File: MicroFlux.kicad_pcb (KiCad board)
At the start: 2 copper layers, 30.5 x 53.3 mm, 24 parts, among them J1 Audio Out, J2 Audio In, U1 LM358

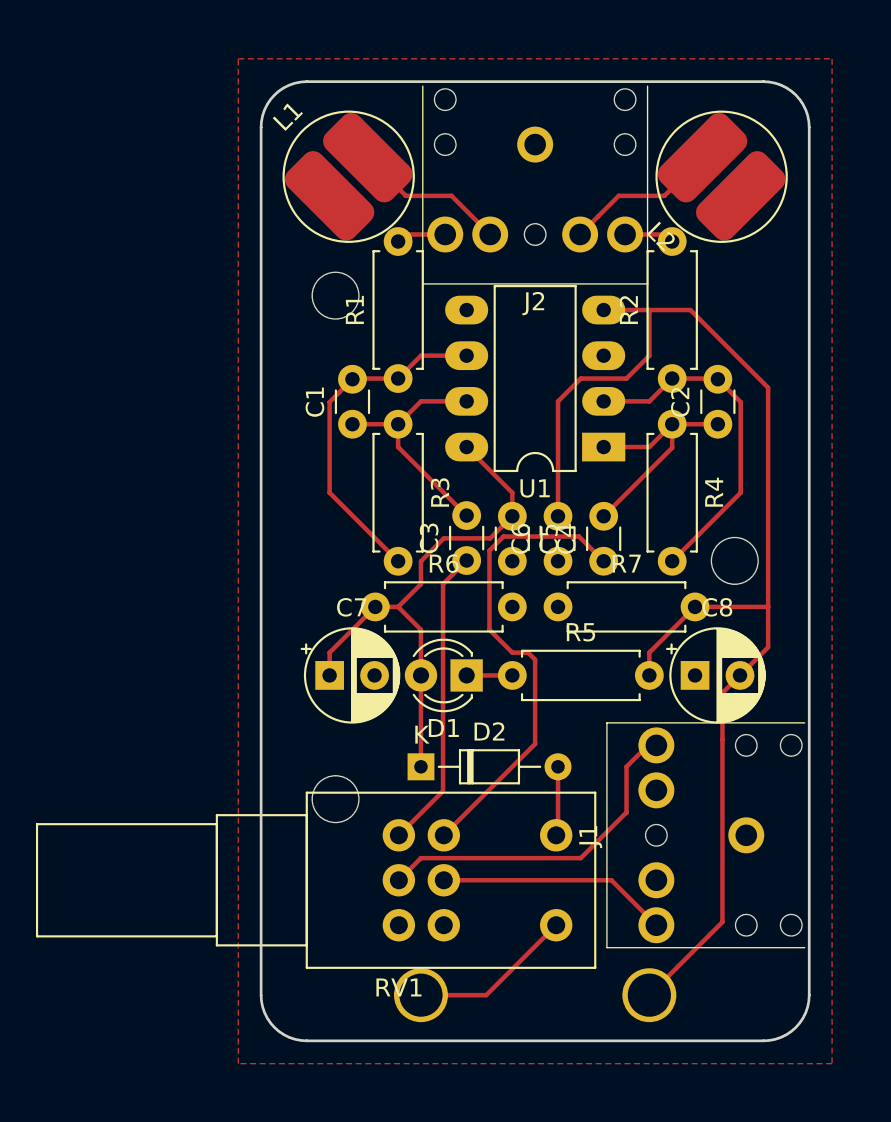
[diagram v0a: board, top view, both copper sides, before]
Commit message: betterplace an route
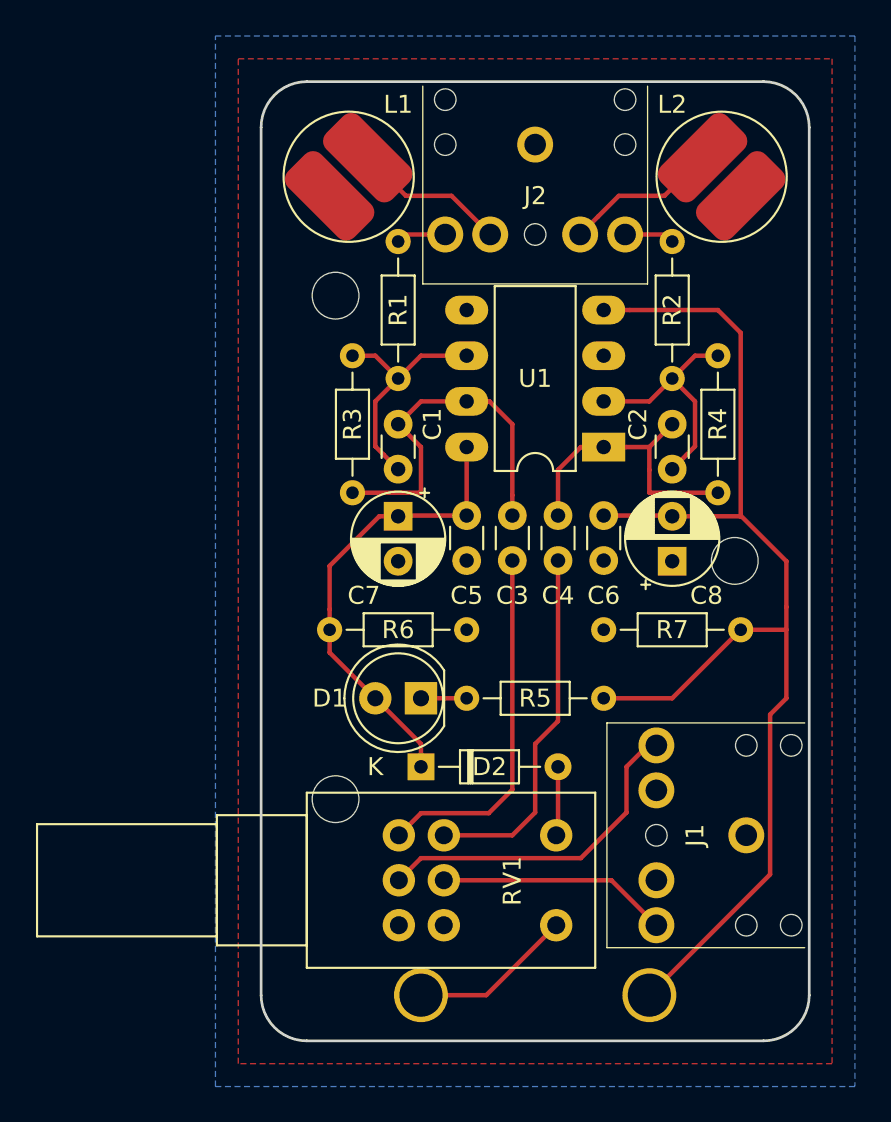
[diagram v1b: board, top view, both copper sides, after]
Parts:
- D1: footprint LED_THT:LED_D3.0mm -> LED_THT:LED_D5.0mm
- R1, R2, R3, R4, R5, R6, R7: footprint Resistor_THT:R_Axial_DIN0207_L6.3mm_D2.5mm_P7.62mm_Horizontal -> Resistor_THT:R_Axial_DIN0204_L3.6mm_D1.6mm_P7.62mm_Horizontal
- moved C7 9.64 mm to (176.5, 87.7), turned to 270 degrees
- moved C8 6.48 mm to (191.8, 90.2), turned to 90 degrees
- moved R3 4.58 mm to (174.0, 86.4), turned to 90 degrees
- moved R4 4.58 mm to (194.3, 86.4), turned to 90 degrees
- moved R7 2.84 mm to (188.0, 94.0)
- moved D1 2.84 mm to (177.8, 97.8)
- moved R5 2.84 mm to (180.3, 97.8)
- moved R6 2.84 mm to (172.7, 94.0)
- moved C4 2.54 mm to (185.4, 90.1)
- moved C6 2.54 mm to (188.0, 90.1)
- moved C5 2.54 mm to (180.3, 87.6)
- moved C1 2.54 mm to (176.5, 82.5), turned to 270 degrees
- moved C2 2.54 mm to (191.8, 82.5), turned to 270 degrees
- moved C3 2.54 mm to (182.9, 90.1)
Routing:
- net AMPLIFIED_LEFT: track 13.5 -> 20.6 mm
- net Net-(C4-Pad1): track 26.7 -> 20.1 mm
- net Net-(C2-Pad2): track 19.1 -> 13.5 mm
- net Net-(C1-Pad2): track 19.1 -> 13.5 mm
- net +BATT: track 29.6 -> 25.9 mm
- net Net-(C3-Pad1): track 16.8 -> 20.1 mm
- net -BATT: track 71.4 -> 68.6 mm
- net AMPLIFIED_RIGHT: track 13.6 -> 16.3 mm
- added copper zone on B.Cu, net (none)
